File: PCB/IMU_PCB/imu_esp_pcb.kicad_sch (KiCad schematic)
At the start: 22 parts, among them J1 Conn_01x02_Pin, J2 Conn_01x05_Pin, U2 ESP32-C3-WROOM-02, U3 PTS647SM38SMTR2LFS, U4 XC6206P332MR-G, U5 1N5819HW-7-F, U6 BMI270

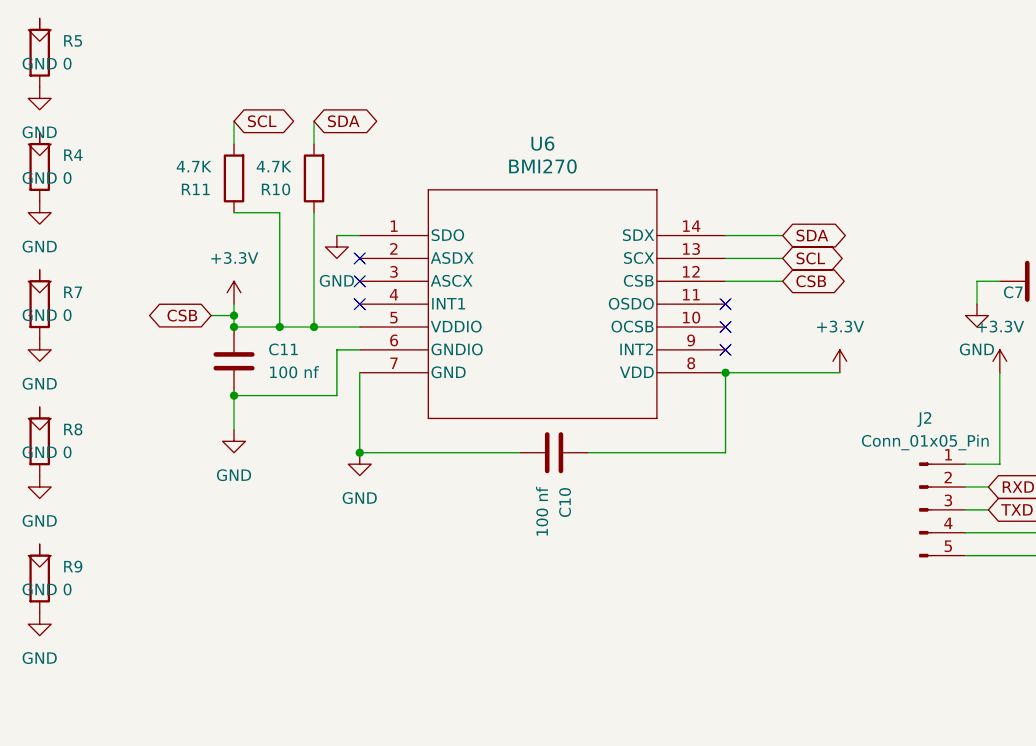
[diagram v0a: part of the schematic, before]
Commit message: PCB for IMU
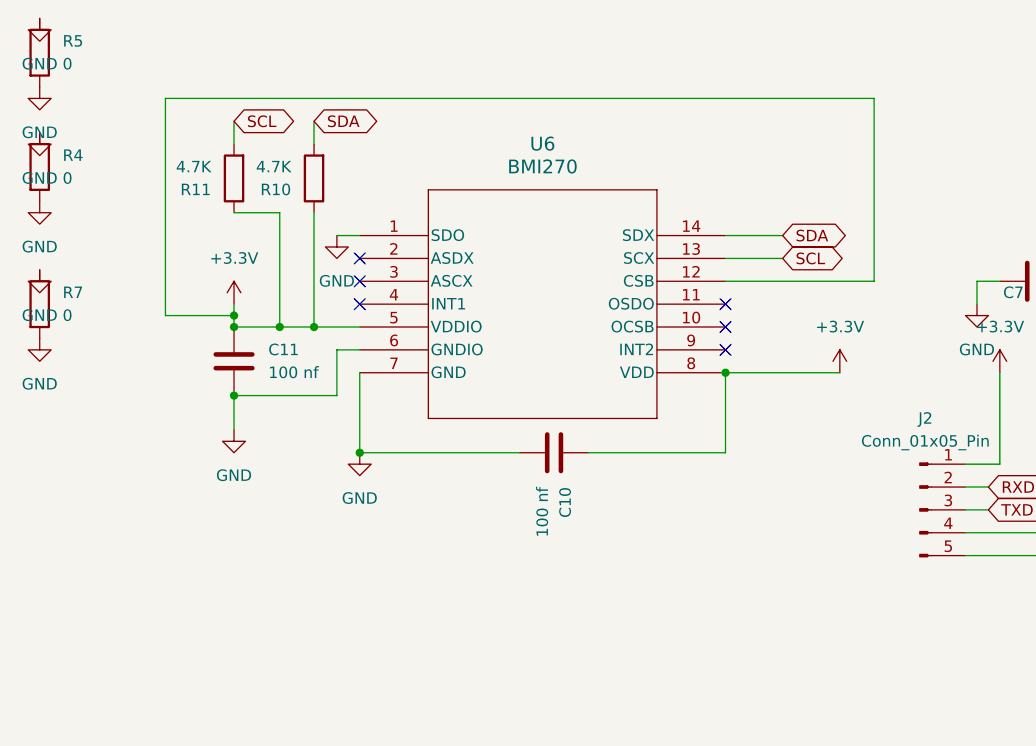
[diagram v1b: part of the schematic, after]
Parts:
- removed R8, R9: 0, Resistor_SMD:R_0805_2012Metric_Pad1.20x1.40mm_HandSolder, symbol Device:R
